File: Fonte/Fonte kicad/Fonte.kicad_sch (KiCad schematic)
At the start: 45 parts, among them J2 Screw_Terminal_01x01, J2 Screw_Terminal_01x03, K2 Relay_SPDT, Q1 BC547, Q2 BC556, Q3 BC556, Q4 IRF540N, Q5 2N7000, Q6 BC547, U1 LM324, U2 LM324, U3 LM324

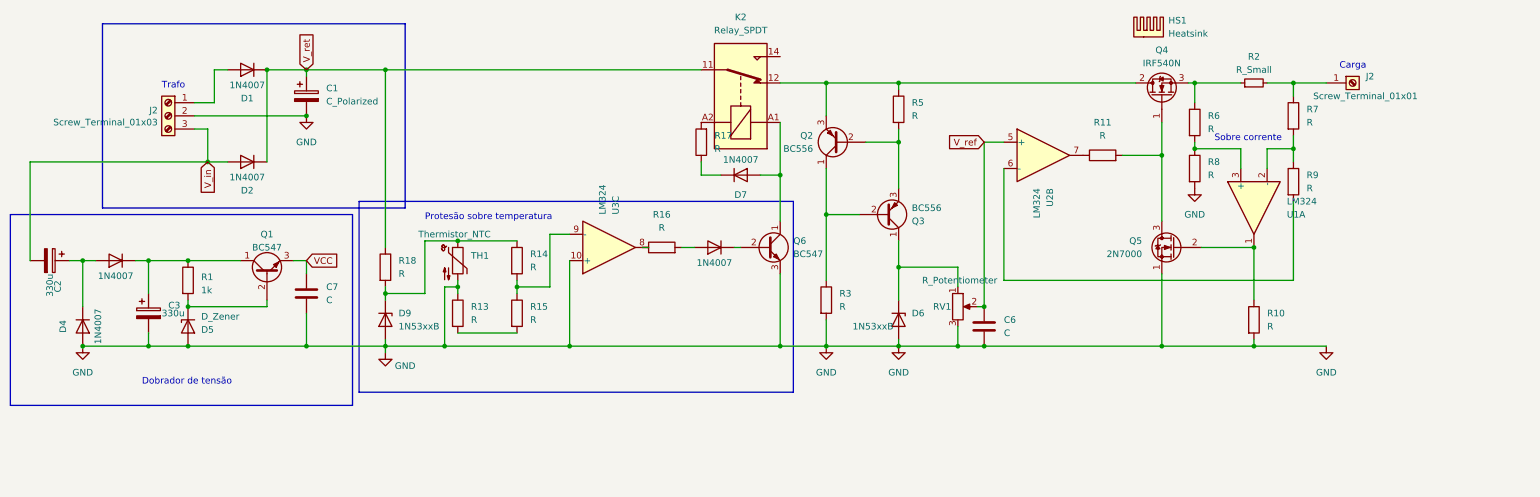
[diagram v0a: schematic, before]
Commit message: Add files via upload
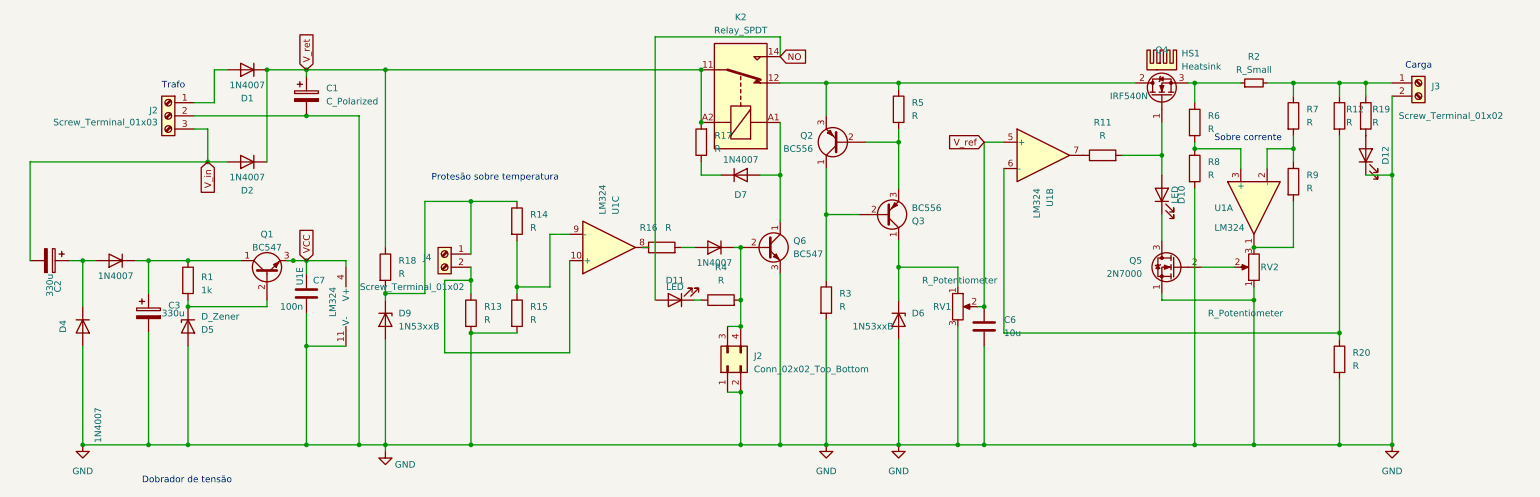
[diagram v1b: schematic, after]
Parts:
- removed J2: Screw_Terminal_01x01, symbol Connector:Screw_Terminal_01x01
- removed R10: R, symbol Device:R
- removed TH1: Thermistor_NTC, symbol Device:Thermistor_NTC
- added D10, D11, D12: LED, LED_THT:LED_D5.0mm, symbol Device:LED
- added J2: Conn_02x02_Top_Bottom, Package_DIP:DIP-4_W10.16mm, symbol Connector_Generic:Conn_02x02_Top_Bottom
- added J3, J4: Screw_Terminal_01x02, TerminalBlock_Phoenix:TerminalBlock_Phoenix_MKDS-1,5-2_1x02_P5.00mm_Horizontal, symbol Connector:Screw_Terminal_01x02
- added R12, R19, R20, R4: R, Resistor_THT:R_Axial_DIN0207_L6.3mm_D2.5mm_P10.16mm_Horizontal, symbol Device:R
- added RV2: R_Potentiometer, Potentiometer_THT:Potentiometer_Piher_PC-16_Single_Horizontal, symbol Device:R_Potentiometer
- added unit 5 of U1
- C1: footprint Capacitor_THT:CP_Radial_D30.0mm_P10.00mm_SnapIn -> Capacitor_THT:CP_Radial_D22.0mm_P10.00mm_SnapIn
- C2, C3: footprint Capacitor_THT:CP_Axial_L18.0mm_D6.5mm_P25.00mm_Horizontal -> Capacitor_THT:CP_Radial_D12.5mm_P5.00mm
- C6: value C -> 10u; footprint (none) -> Capacitor_THT:CP_Radial_D10.0mm_P7.50mm
- C7: value C -> 100n; footprint (none) -> Capacitor_THT:CP_Radial_D10.0mm_P7.50mm
- D5: footprint Diode_THT:D_DO-201AD_P12.70mm_Horizontal -> Diode_THT:D_DO-41_SOD81_P10.16mm_Horizontal
- D6, D9: footprint Diode_THT:D_DO-201_P15.24mm_Horizontal -> Diode_THT:D_DO-41_SOD81_P10.16mm_Horizontal
- HS1: footprint (none) -> Heatsink:Heatsink_Stonecold_HS-132_32x14mm_2xFixation1.5mm
- K2: footprint (none) -> Relay_THT:Relay_SPDT_Finder_40.31
- R1: footprint Resistor_THT:R_Axial_DIN0918_L18.0mm_D9.0mm_P7.62mm_Vertical -> Resistor_THT:R_Axial_DIN0207_L6.3mm_D2.5mm_P10.16mm_Horizontal
- R11, R13, R14, R15, R16, R17, R18, R3, R5, R6, R7, R8, R9: footprint (none) -> Resistor_THT:R_Axial_DIN0207_L6.3mm_D2.5mm_P10.16mm_Horizontal
- R2: footprint (none) -> Diode_THT:D_P600_R-6_P20.00mm_Horizontal
- RV1: footprint Potentiometer_SMD:Potentiometer_ACP_CA6-VSMD_Vertical -> Potentiometer_THT:Potentiometer_Piher_PC-16_Single_Horizontal
- U1: footprint (none) -> Package_DIP:DIP-14_W7.62mm
- U1: renamed from U2; footprint (none) -> Package_DIP:DIP-14_W7.62mm
- U1: renamed from U3; footprint (none) -> Package_DIP:DIP-14_W7.62mm
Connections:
- net GND: now also R13.2, R15.2, D12.1 (K), J2.1 (Pin_1), J2.2 (Pin_2), J3.2 (Pin_2), R20.2, RV2.1, U1.11 (V-); no longer R13.1, U1.10 (+)
- net VCC: now also U1.4 (V+)
- net V_ret: now also K2.A2, R17.2
- net at Q4.1 (G), R11.2: now also D10.2 (A); no longer Q5.3 (D)
- net at R9.2: now also U1.1, RV2.3; no longer U1.6 (-)
- net at D8.1 (K), Q6.2 (B): now also J2.3 (Pin_3), J2.4 (Pin_4), R4.2
- net at R2.2, R7.1: now also J3.1 (Pin_1), R12.1, R19.1
- net at D9.1 (K), R14.1, R18.2: now also J4.1 (Pin_1)
- net at Q5.2 (G): now also RV2.2; no longer U1.1
- net NO: now reaches K2.14
- net NO: now also D11.2 (A)
- new net: J4.2 (Pin_2), R13.1, U1.10 (+)
- new net: D10.1 (K), Q5.3 (D)
- new net: D12.2 (A), R19.2
- new net: R12.2, R20.1, U1.6 (-)
- new net: D11.1 (K), R4.1
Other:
- moved on the sheet: HS1, Q5, R13, R14
